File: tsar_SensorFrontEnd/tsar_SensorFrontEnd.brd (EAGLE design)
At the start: 150.1 x 82.7 mm, 108 parts, among them J1 IDC_RECEPTACLE_2X20-S9175-ND

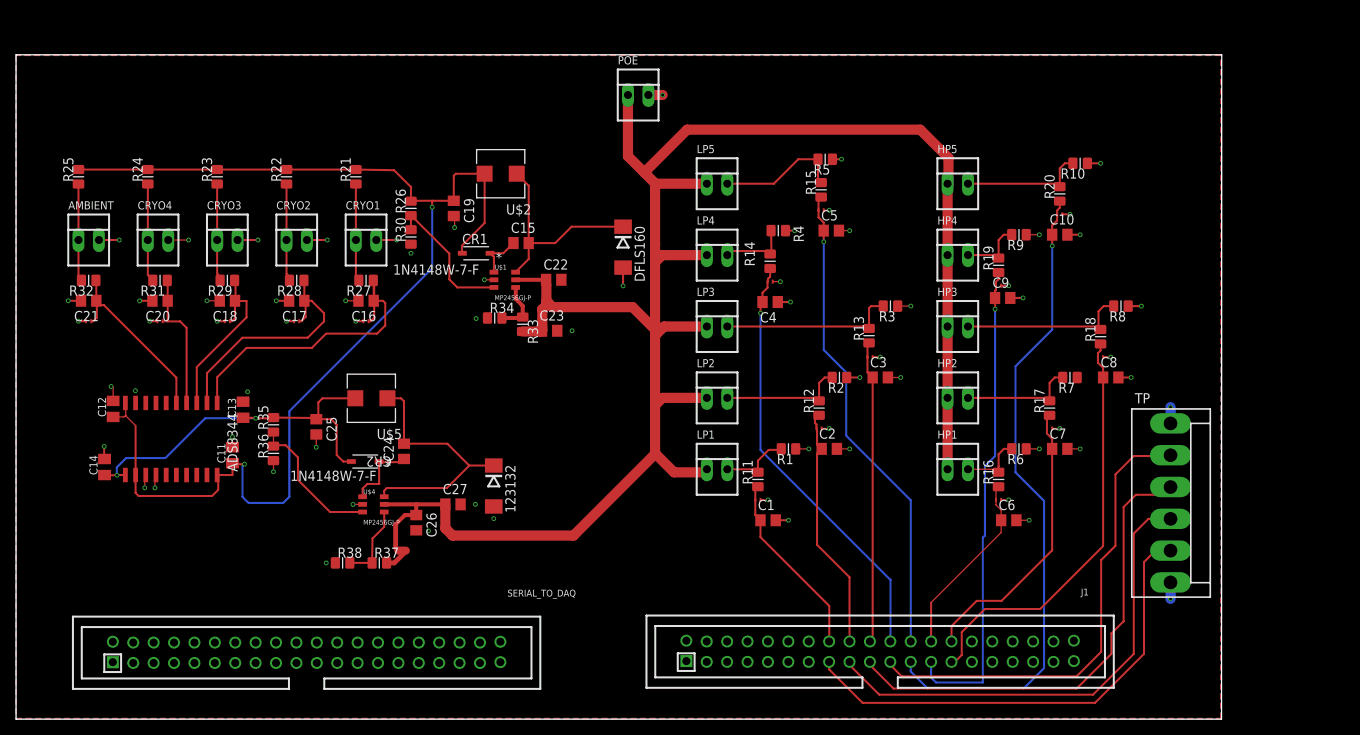
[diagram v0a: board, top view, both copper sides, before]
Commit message: ADS connected
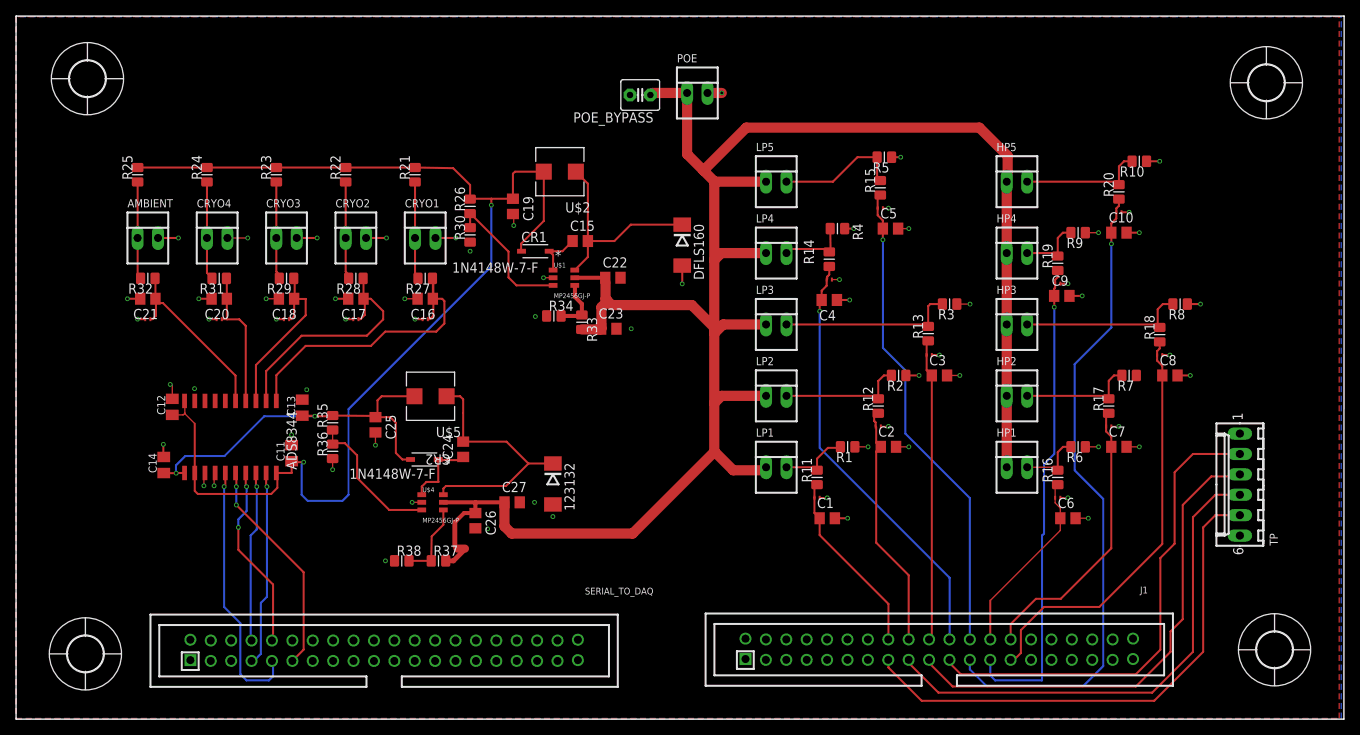
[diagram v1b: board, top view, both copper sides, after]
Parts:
- added H1, H2, H3, H4: MOUNT-HOLE4.5, holes:4,5
- added POE_BYPASS: 100u, capacitor-wima:C2.5-4
- R33, R37: value 500k -> 10k
- R34, R38: value TBD -> NP
- TP: value (none) -> 22-27-2061-06; device con-molex:KK-156-6 -> con-molex:6410-06
- moved SERIAL_TO_DAQ 9.66 mm to (45.8, 8.52)
- moved TP 8.93 mm to (152.4, 29.2), turned to 90 degrees
- moved C8 7.37 mm to (143.7, 42.8)
- moved R16 7.37 mm to (129.7, 30.1)
- moved R17 7.37 mm to (136.1, 39.0)
- moved R18 7.37 mm to (142.4, 47.9)
- moved R19 7.37 mm to (129.7, 56.8)
- moved TVS6 7.37 mm to (129.7, 27.6)
- moved TVS7 7.37 mm to (136.1, 36.4)
- moved TVS8 7.37 mm to (142.4, 45.3)
- moved TVS9 7.37 mm to (129.7, 54.2)
- moved R10 7.37 mm to (139.9, 69.5)
- moved CR1 7.37 mm to (64.7, 58.3)
- moved R34 7.37 mm to (67.0, 50.2)
- moved C13 7.37 mm to (35.6, 38.8)
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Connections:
- new net N$11: SERIAL_TO_DAQ.7, U$3.19
- new net N$13: SERIAL_TO_DAQ.10, U$3.17
- new net N$17: SERIAL_TO_DAQ.9, U$3.15
- new net N$18: SERIAL_TO_DAQ.8, U$3.18
- new net N$20: SERIAL_TO_DAQ.11, U$3.16
- net +12V: now also POE_BYPASS.1
- net GND: now also POE_BYPASS.2
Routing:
- net N$17: track 0.00 -> 32.5 mm, vias 0 -> 1
- net N$20: track 0.00 -> 27.5 mm, vias 0 -> 2
- net N$11: track 0.00 -> 24.4 mm, vias 0 -> 1
- net N$13: track 0.00 -> 23.2 mm, vias 0 -> 2
- net N$18: track 0.00 -> 21.3 mm, vias 0 -> 1
- net N$12: track 59.7 -> 65.1 mm
- net GND: track 87.8 -> 83.0 mm, vias 67 -> 65
- net +12V: track 242.1 -> 246.8 mm
- net N$16: track 59.7 -> 63.2 mm
- net N$14: track 59.2 -> 61.1 mm
- net N$15: track 59.2 -> 60.4 mm
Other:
- board size 150.1 x 82.7 mm -> 165.4 x 87.6 mm

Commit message: I broke everything
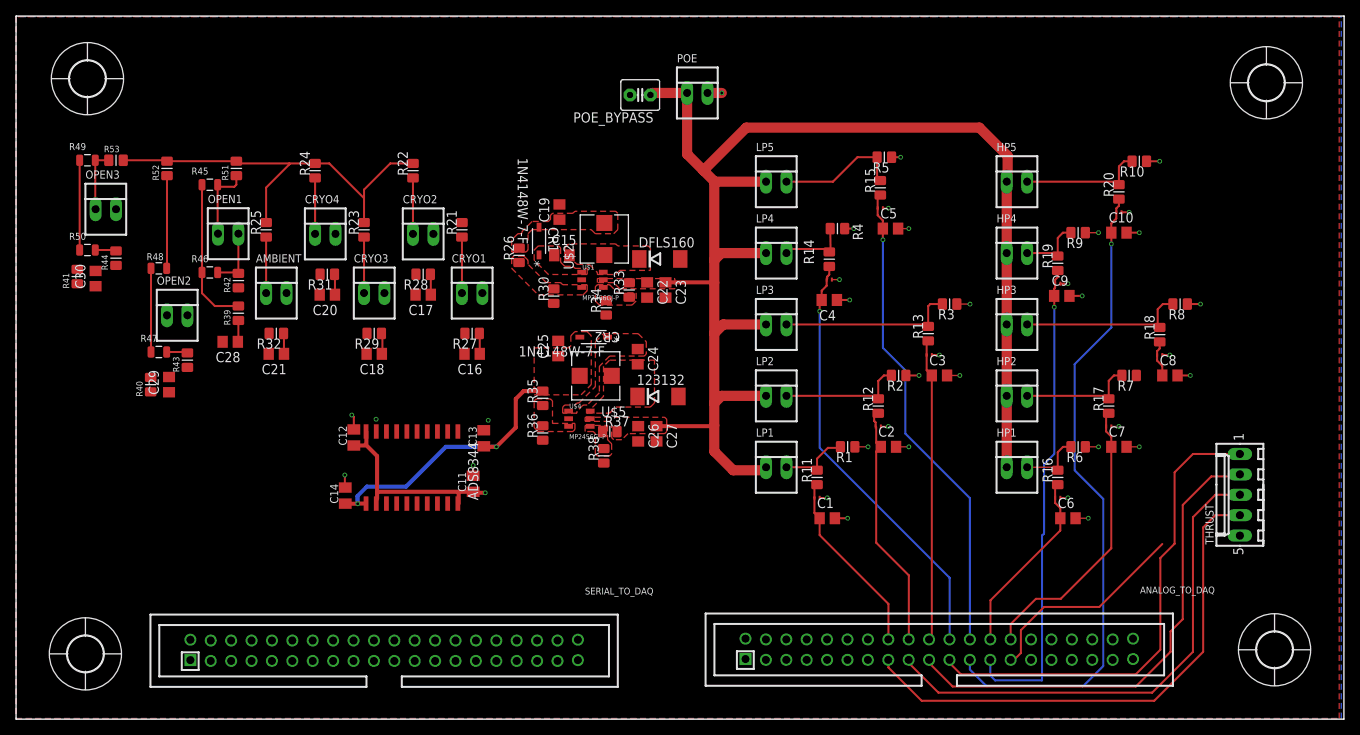
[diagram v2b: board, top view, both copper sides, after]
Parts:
- removed TP: 22-27-2061-06, con-molex:6410-06
- removed TVS12, TVS13, TVS14, TVS16, TVS17: DF2B5M4CT,L3F, TSAR_Controller:SOD-882(SOT2)
- added C28, C29, C30: 120pF, rcl:C0805
- added OPEN1, OPEN2, OPEN3: 22-23-2021, con-molex:22-23-2021
- added R39, R40, R41, R42, R43, R44: 1k, marionette:.0805-B
- added R45, R46, R47, R48, R49, R50: NP, Resistor_Capacitor:RES_0805
- added R51, R52, R53: 150, marionette:.0805-B
- added THRUST: Thrust Plate Connector, con-molex:6410-05
- R25: value 150 -> 22k
- R35: value TBD -> 73.2k
- R36: value TBD -> 23.7k
- moved R38 28.4 mm to (73.2, 32.8), turned to 90 degrees
- moved R37 26.7 mm to (73.9, 35.8)
- moved R35 26.3 mm to (65.6, 40.0)
- moved R36 26.3 mm to (65.6, 35.6)
- moved CR2 26.0 mm to (71.9, 47.6)
- moved C25 24.7 mm to (67.5, 46.2), turned to 90 degrees
- moved C24 24.6 mm to (77.4, 45.1), turned to 270 degrees
- moved C26 23.0 mm to (77.5, 35.5)
- moved C11 22.9 mm to (56.9, 29.3)
- moved C14 22.9 mm to (41.0, 27.8)
- moved U$3 22.9 mm to (49.3, 31.3)
- moved C12 22.9 mm to (42.1, 35.1)
- moved C13 22.9 mm to (58.2, 35.0)
- moved U$4 21.0 mm to (70.2, 37.4)
- moved U$5 20.7 mm to (72.2, 42.7)
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- renumbered J1 to ANALOG_TO_DAQ
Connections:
- removed net 14: C16.1, R27.1, TVS12.P$1, U$3.1
- removed net 15: C17.1, R28.1, TVS13.P$1, U$3.2
- removed net 16: C18.1, R29.1, TVS14.P$1, U$3.3
- removed net 18: C20.1, R31.1, TVS16.P$1, U$3.4
- new net 11: C28.1, R39.1, U$3.6
- new net 12: C29.1, R40.1, U$3.7
- new net 13: C30.1, R41.1, U$3.8
- new net N$21: C16.1, R27.1, U$3.1
- new net N$23: C17.1, R28.1, U$3.2
- new net N$24: C18.1, R29.1, U$3.3
- new net N$25: C20.1, R31.1, U$3.4
- new net N$26: OPEN1.2, R42.2, R46.2
- new net N$27: OPEN2.2, R43.2, R47.2
- new net N$28: OPEN3.2, R44.2, R50.2
- new net N$30: R40.2, R47.1, R48.1
- new net N$31: R41.2, R49.1, R50.1
- new net N$32: R39.2, R45.1, R46.1
- new net N$33: OPEN3.1, R49.2, R53.1
- new net N$34: OPEN2.1, R48.2, R52.1
- new net N$35: OPEN1.1, R45.2, R51.1
- net +5V: now also R51.2, R52.2, R53.2
- net 19: no longer TVS17.P$1
- net GND: now also C28.2, C29.2, C30.2, R42.1, R43.1, R44.1, THRUST.5; no longer TP.1, TP.6, TVS12.P$2, TVS13.P$2, TVS14.P$2, TVS16.P$2, TVS17.P$2
- net N$12: now also THRUST.4; no longer TP.5
- net N$14: now also THRUST.2; no longer TP.3
- net N$15: now also THRUST.1; no longer TP.2
- net N$16: now also THRUST.3; no longer TP.4
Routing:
- net +5V: track 153.3 -> 77.9 mm, vias 2 -> 1
- net +12V: track 246.8 -> 179.2 mm
- net 14: track 39.2 -> 0.00 mm
- net GND: track 83.0 -> 45.5 mm, vias 65 -> 35
- net N$17: track 32.5 -> 0.00 mm, vias 1 -> 0
- net GND2: track 32.5 -> 0.00 mm
- net 15: track 30.7 -> 0.00 mm
- net N$20: track 27.5 -> 0.14 mm, vias 2 -> 0
- net GND1: track 26.1 -> 0.00 mm
- net N$11: track 24.4 -> 0.00 mm, vias 1 -> 0
- net N$13: track 23.2 -> 0.00 mm, vias 2 -> 0
- net 16: track 22.3 -> 0.00 mm
- net N$18: track 21.3 -> 0.00 mm, vias 1 -> 0
- net 8: track 52.1 -> 31.1 mm
- net 19: track 22.9 -> 3.67 mm
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- added copper zone on layer 1, net +12V
- added copper zone on layer 1, net +3V3
- added copper zone on layer 1, net +5V
- added copper zone on layer 1, net GND1
- added copper zone on layer 1, net GND2
- added copper zone on layer 1, net N$10
- added copper zone on layer 1, net N$3
- added copper zone on layer 1, net N$4
- added copper zone on layer 1, net N$5
- added copper zone on layer 1, net N$8
- added copper zone on layer 1, net N$9
